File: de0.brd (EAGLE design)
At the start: 149.9 x 88.9 mm, 137 parts, among them IC1 PL2303SA__LF, J1 JUMPER_IN_50, J2 UX60SC-MB-5ST, J3 REG_OUT_33, U1 P0082, U2 RFM95W-915S2, U3 TPS76201DBVR, U4 TPS76201DBVR, U5 TPS76201DBVR

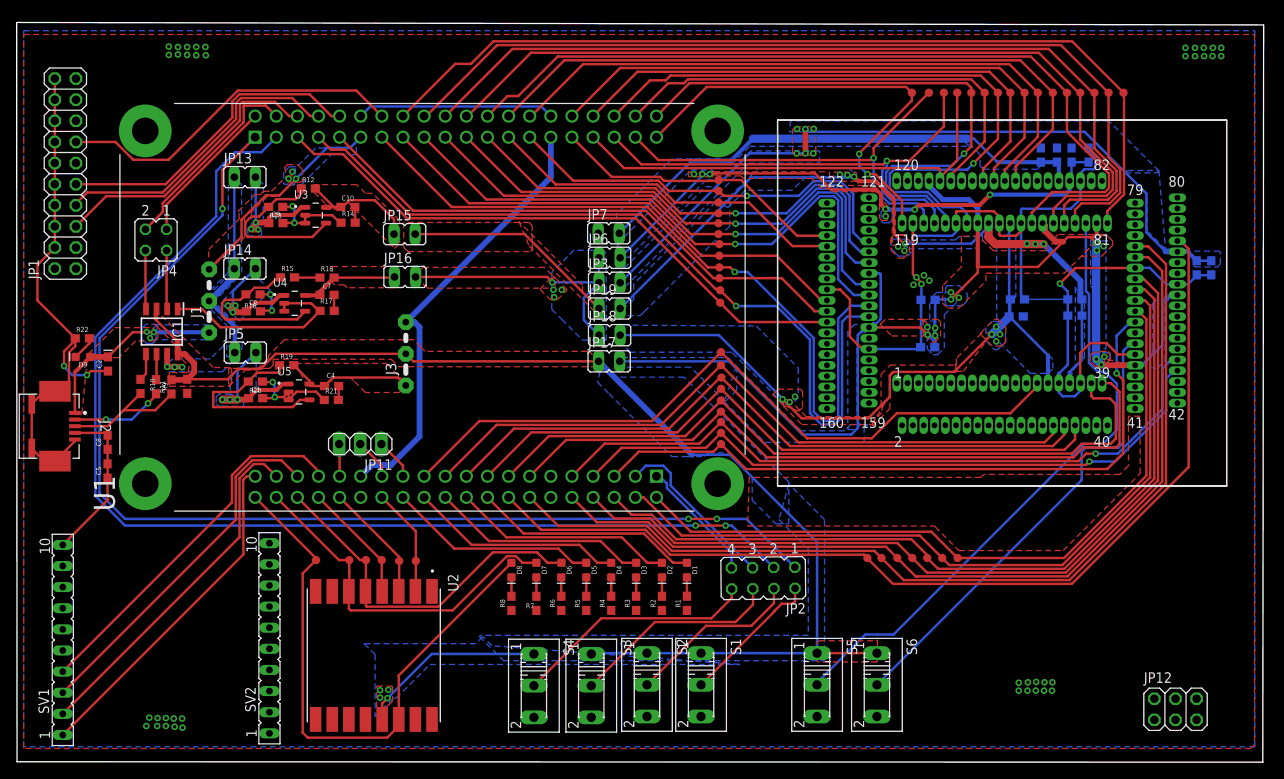
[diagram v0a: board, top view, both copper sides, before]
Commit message: Organize the schematic and the layout
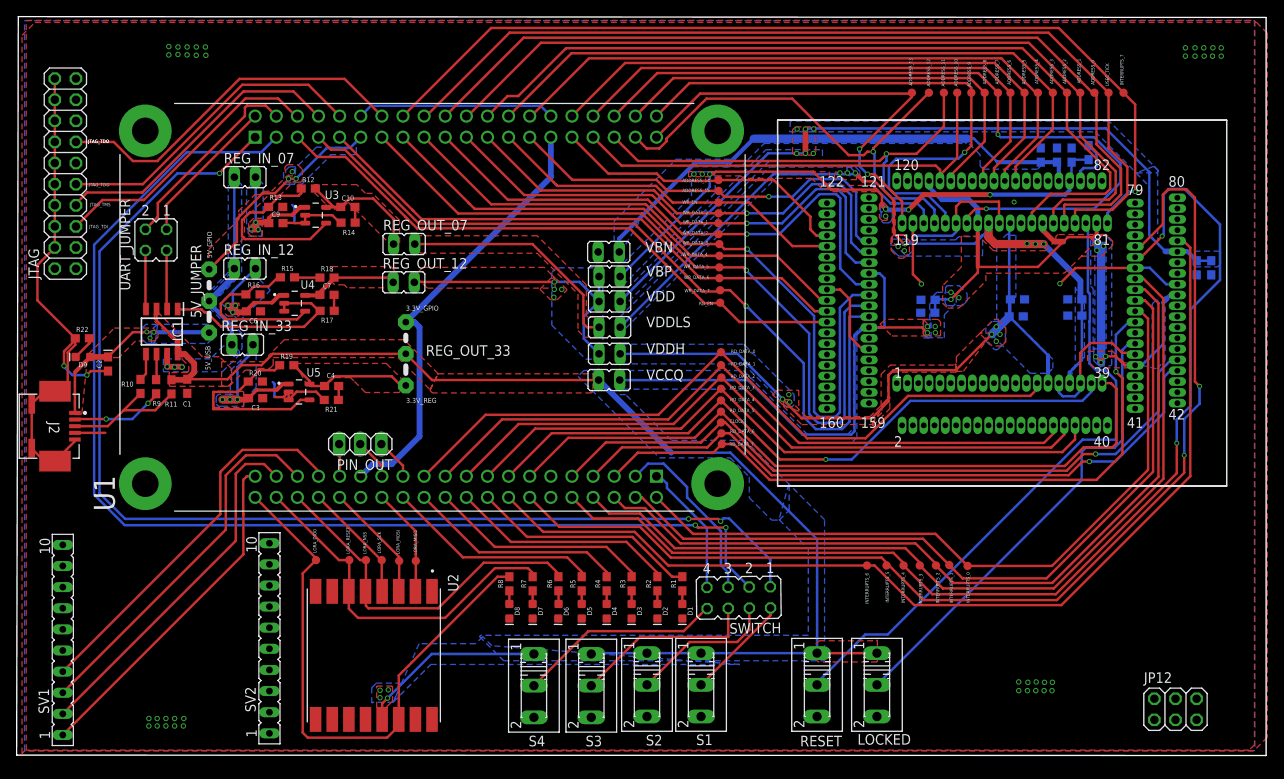
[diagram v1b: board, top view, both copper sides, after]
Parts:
- removed C5, C8: 1nF, SparkFun-Capacitors:0603
- removed JP15: REG_OUT_07, jumper:JP1
- removed JP16: REG_OUT_12, jumper:JP1
- removed JP17: VCCQ, jumper:JP1
- removed JP18: VDDH, jumper:JP1
- removed JP19: VDDLS, jumper:JP1
- removed JP2: SWITCH, jumper:JP4Q
- removed JP3: VDD, jumper:JP1
- removed JP5: REG_IN_33, jumper:JP1
- removed JP6: VBP, jumper:JP1
- removed JP7: VBN, jumper:JP1
- removed U$16: INTERRUPTS_6, qfp160:POINT
- added INTERRUPTS_6: INTERRUPTS_6, qfp160:POINT
- added REG_IN_33: REG_IN_33, jumper:JP1
- added REG_OUT_07: REG_OUT_07, jumper:JP1
- added REG_OUT_12: REG_OUT_12, jumper:JP1
- added SWITCH: SWITCH, jumper:JP4Q
- added VBN: VBN, jumper:JP1
- added VBP: VBP, jumper:JP1
- added VCCQ: VCCQ, jumper:JP1
- added VDD: VDD, jumper:JP1
- added VDDH: VDDH, jumper:JP1
- added VDDLS: VDDLS, jumper:JP1
- moved D1 4.98 mm to (14.7, -16.8)
- moved D2 4.98 mm to (11.7, -16.8)
- moved D3 4.98 mm to (8.55, -16.8)
- moved D4 4.98 mm to (5.55, -16.8)
- moved D5 4.98 mm to (2.55, -16.8)
- moved D7 4.97 mm to (-3.35, -16.8)
- moved D6 4.96 mm to (-0.25, -16.8)
- moved D8 4.96 mm to (-6.15, -16.8)
- moved C12 4.14 mm to (44.2, 19.1)
- moved R4 2.41 mm to (5.55, -13.4)
- moved R5 2.41 mm to (2.55, -13.4)
- moved R1 2.41 mm to (14.7, -13.4)
- moved R2 2.41 mm to (11.7, -13.4)
- moved R3 2.41 mm to (8.55, -13.4)
- moved R7 2.39 mm to (-3.35, -13.4)
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- renumbered J1 to 5V_JUMPER, J3 to REG_OUT_33, JP1 to JTAG, JP11 to PIN_OUT, JP13 to REG_IN_07, JP14 to REG_IN_12, JP4 to UART_JUMPER, S5 to RESET, S6 to LOCKED
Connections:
- net N$18 renamed D-
- net N$19 renamed D+
- removed net N$13: JP2.2, S1.2
- removed net N$14: JP2.4, S2.2
- removed net N$15: JP2.6, S3.2
- removed net N$16: JP2.8, S4.2
- removed net N$24: JP2.5, U1.JP2_3
- new net GPIO0_IN_0: SWITCH.1, U1.JP1_1
- new net GPIO0_IN_1: SWITCH.3, U1.JP1_3
- new net GPIO1_IN_0: SWITCH.7, U1.JP2_1
- new net GPIO1_IN_1: SWITCH.5, U1.JP2_3
- new net N$12: S1.2, SWITCH.2
- net GND: now also D1.C, D2.C, D3.C, D4.C, D5.C, D6.C, D7.C, D8.C, VBN.1; no longer C5.1, C5.2, C8.1, C8.2, JP7.1, R1.1, R2.1, R3.1, R4.1, R5.1, R6.1, R7.1, R8.1
- net GPIO_OUT_0: now also R1.2; no longer D1.A
- net GPIO_OUT_1: now also R2.2; no longer D2.A
- net GPIO_OUT_2: now also R3.2; no longer D3.A
- net GPIO_OUT_3: now also R4.2; no longer D4.A
- net GPIO_OUT_4: now also R5.2; no longer D5.A
- net INTERRUPTS_6: now also INTERRUPTS_6.1; no longer U$16.1
- net IN_33: now also REG_IN_33.2; no longer JP5.2
- net LORA_DIO0: now also R8.2; no longer D8.A
- net LORA_NSS: now also R6.2; no longer D6.A
- net LORA_RESET: now also R7.2; no longer D7.A
- net N$1: now also D1.A, R1.1; no longer D1.C, R1.2
- net N$10: now also S3.2, SWITCH.6; no longer JP2.3, U1.JP1_3
- net N$11: now also S2.2, SWITCH.4; no longer JP2.7, U1.JP2_1
- net N$2: now also D8.A, R8.1; no longer D2.C, R2.2
- net N$3: now also D7.A, R7.1; no longer D3.C, R3.2
- net N$4: now also D6.A, R6.1; no longer D4.C, R4.2
- net N$5: now also D5.A, R5.1; no longer D5.C, R5.2
- net N$6: now also D4.A, R4.1; no longer D6.C, R6.2
- net N$7: now also D2.A, R2.1; no longer D7.C, R7.2
- net N$8: now also D3.A, R3.1; no longer D8.C, R8.2
- net N$9: now also S4.2, SWITCH.8; no longer JP2.1, U1.JP1_1
- net OUT_07: now also REG_OUT_07.1; no longer JP15.1
- net OUT_12: now also REG_OUT_12.1; no longer JP16.1
- net VBN: now also VBN.2; no longer JP7.2
- net VBP: now also VBP.2; no longer JP6.2
- net VCCQ: now also VCCQ.2; no longer JP17.2
- net VDD: now also VDD.2; no longer JP3.2
- net VDD5: now also REG_IN_33.1; no longer JP5.1
- net VDDH: now also VDDH.2; no longer JP18.2
- net VDDLS: now also VDDLS.2; no longer JP19.2
- net VO_07: now also REG_OUT_07.2, VDDLS.1; no longer JP15.2, JP19.1
- net VO_12: now also REG_OUT_12.2, VBP.1, VDD.1, VDDH.1; no longer JP16.2, JP18.1, JP3.1, JP6.1
- net VO_33: now also VCCQ.1; no longer JP17.1
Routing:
- net GPIO0_IN_1: track 0.00 -> 143.2 mm, vias 0 -> 2
- net GPIO0_IN_0: track 0.00 -> 141.1 mm, vias 0 -> 3
- net N$10: track 139.1 -> 22.3 mm, vias 2 -> 0
- net N$9: track 137.9 -> 24.7 mm, vias 3 -> 0
- net GND: track 298.9 -> 214.2 mm, vias 54 -> 45
- net N$16: track 29.2 -> 0.00 mm
- net N$15: track 25.4 -> 0.00 mm
- net INTERRUPTS_4: track 108.9 -> 134.0 mm, vias 0 -> 2
- net GPIO1_IN_1: track 0.00 -> 22.1 mm
- net N$14: track 21.1 -> 0.00 mm
- net N$24: track 20.6 -> 0.00 mm
- net INTERRUPTS_5: track 116.4 -> 136.9 mm, vias 0 -> 2
- net N$13: track 17.0 -> 0.00 mm
- net GPIO1_IN_0: track 0.00 -> 16.1 mm
- net WR_DATA_3: track 71.7 -> 87.6 mm
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- added copper zone on layer 1, net IN_07
- added copper zone on layer 1, net IN_12
- added copper zone on layer 1, net IN_33
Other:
- board size 149.9 x 88.9 mm -> 150.2 x 88.8 mm
- board text added: "3.3V_GPIO"
- board text added: "3.3V_REG"
- board text added: "5V_GPIO"
- board text added: "5V_USB"
- board text added: "ADDRESS_0"
- board text added: "ADDRESS_1"
- board text added: "ADDRESS_10"
- board text added: "ADDRESS_11"
- board text added: "ADDRESS_12"
- board text added: "ADDRESS_13"
- board text added: "ADDRESS_14"
- board text added: "ADDRESS_15"
- board text added: "ADDRESS_2"
- board text added: "ADDRESS_3"
- board text added: "ADDRESS_4"
- board text added: "ADDRESS_5"
- board text added: "ADDRESS_6"
- board text added: "ADDRESS_7"
- board text added: "ADDRESS_8"
- board text added: "ADDRESS_9"
- board text added: "CLOCK"
- board text added: "INTERRUPTS_0"
- board text added: "INTERRUPTS_1"
- board text added: "INTERRUPTS_2"
- board text added: "INTERRUPTS_3"
- board text added: "INTERRUPTS_4"
- board text added: "INTERRUPTS_5"
- board text added: "INTERRUPTS_6"
- board text added: "INTERRUPTS_7"
- board text added: "JTAG_TDI"
- board text added: "JTAG_TDO"
- board text added: "JTAG_TMS"
- board text added: "LORA_DIO0"
- board text added: "LORA_MISO"
- board text added: "LORA_MOSI"
- board text added: "LORA_NSS"
- board text added: "LORA_RESET"
- board text added: "LORA_SCK"
- board text added: "RD_DATA_0"
- board text added: "RD_DATA_1"
- board text added: "RD_DATA_2"
- board text added: "RD_DATA_3"
- board text added: "RD_DATA_4"
- board text added: "RD_DATA_5"
- board text added: "RD_DATA_6"
- board text added: "RD_DATA_7"
- board text added: "RD_EN"
- board text added: "USEC_TICK"
- board text added: "WR_DATA_0"
- board text added: "WR_DATA_1"
- board text added: "WR_DATA_2"
- board text added: "WR_DATA_3"
- board text added: "WR_DATA_4"
- board text added: "WR_DATA_5"
- board text added: "WR_DATA_6"
- board text added: "WR_DATA_7"
- board text added: "WR_EN"
